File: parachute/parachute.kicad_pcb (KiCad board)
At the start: 2 copper layers, 40 x 30 mm, 16 parts, among them J1 servo, J2 power, J3 hmi, J5 trigger_rpi, J6 trigger_lauch, U1 LTV-814, U3 RP2040, U4 LTV-814

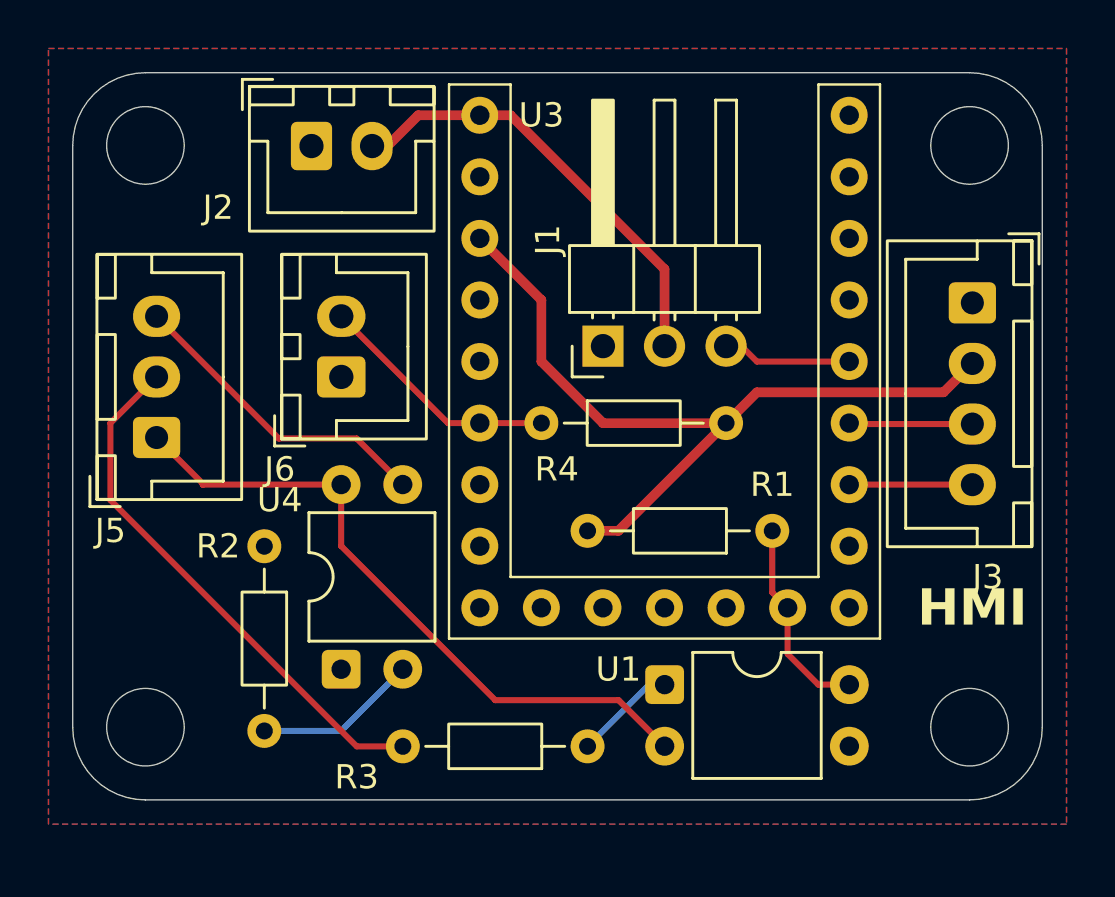
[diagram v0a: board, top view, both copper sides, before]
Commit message: parachute full revision
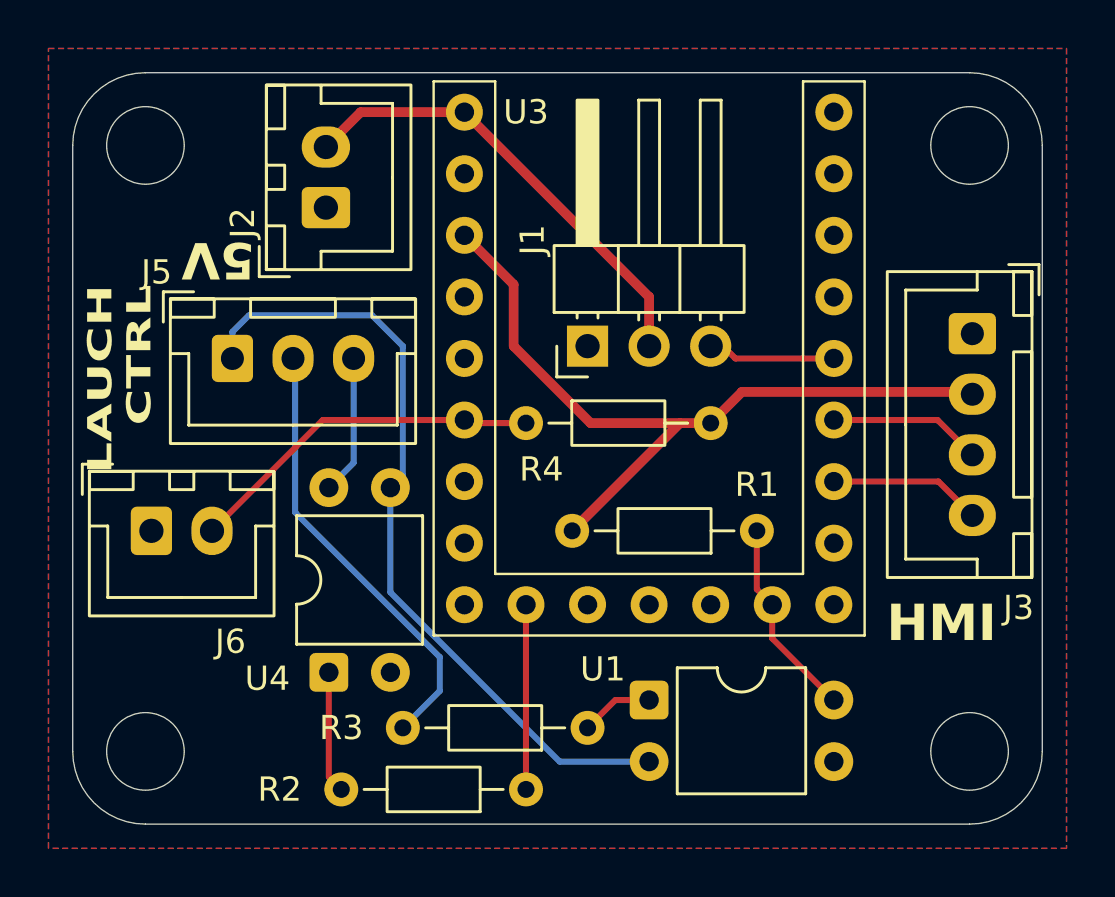
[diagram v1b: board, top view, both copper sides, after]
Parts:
- moved R2 14.7 mm to (139.7, 99.6), turned to 180 degrees
- moved J6 10.1 mm to (124.2, 88.9), turned to 0 degrees
- moved J5 4.52 mm to (127.6, 81.8), turned to 0 degrees
- moved J2 2.61 mm to (131.4, 75.6), turned to 90 degrees
- moved J3 1.27 mm to (158.1, 80.8)
- moved H3 1.00 mm to (124.0, 98.0)
- moved H4 1.00 mm to (158.0, 98.0)
- moved U1 0.90 mm to (144.8, 95.9)
- moved R3 0.76 mm to (142.2, 97.0)
- moved U3 0.65 mm to (144.8, 71.6)
- moved R1 0.64 mm to (149.2, 88.9)
- moved R4 0.64 mm to (139.7, 84.5)
- moved J1 0.63 mm to (142.2, 81.3)
- moved U4 0.52 mm to (131.6, 94.7)
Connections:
- U3 pad 10: unconnected-(U3-GPIO13-Pad10) -> /parachute_open
- U3 pad 8: /parachute_open -> unconnected-(U3-GPIO15-Pad8)
- U4 pad 1: GND -> Net-(R2-Pad2)
- U4 pad 2: Net-(R2-Pad2) -> GND
- U4 pad 3: Net-(J5-Pin_3) -> Net-(J5-Pin_1)
- U4 pad 4: Net-(J5-Pin_1) -> Net-(J5-Pin_3)
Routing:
- net /parachute_open: track 0.00 -> 7.62 mm
- net Net-(J5-Pin_3): track 13.0 -> 5.75 mm
- net Net-(J5-Pin_1): track 27.8 -> 32.9 mm
- net /BUTTON_LAUCHED: track 10.1 -> 14.9 mm
- net Net-(J5-Pin_2): track 22.1 -> 18.4 mm
- net Net-(R2-Pad2): track 6.76 -> 5.04 mm
- net Net-(R3-Pad1): track 4.23 -> 3.02 mm
- net /LED_TIMER_TRIGGED: track 5.08 -> 6.29 mm
- net /LED_OPEN: track 5.10 -> 6.31 mm
- net +3V3: track 33.5 -> 32.5 mm
- net +5V: track 18.4 -> 19.1 mm
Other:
- board size 40 x 30 mm -> 40 x 31 mm
- board text added: "LAUCH CTRL"
- board text removed: "CONTROL"
- board text removed: "LAUCH"
